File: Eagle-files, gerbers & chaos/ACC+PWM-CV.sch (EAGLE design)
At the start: 57 parts, among them IC1 TL072P, Q1 BC546A, Q2 BC556A, Q3 BC546A, Q4 BC546A, Q5 BC546A, Q6 BC546A, X1 ACC+TRIG, X2 OUT, X3 SUPPLY

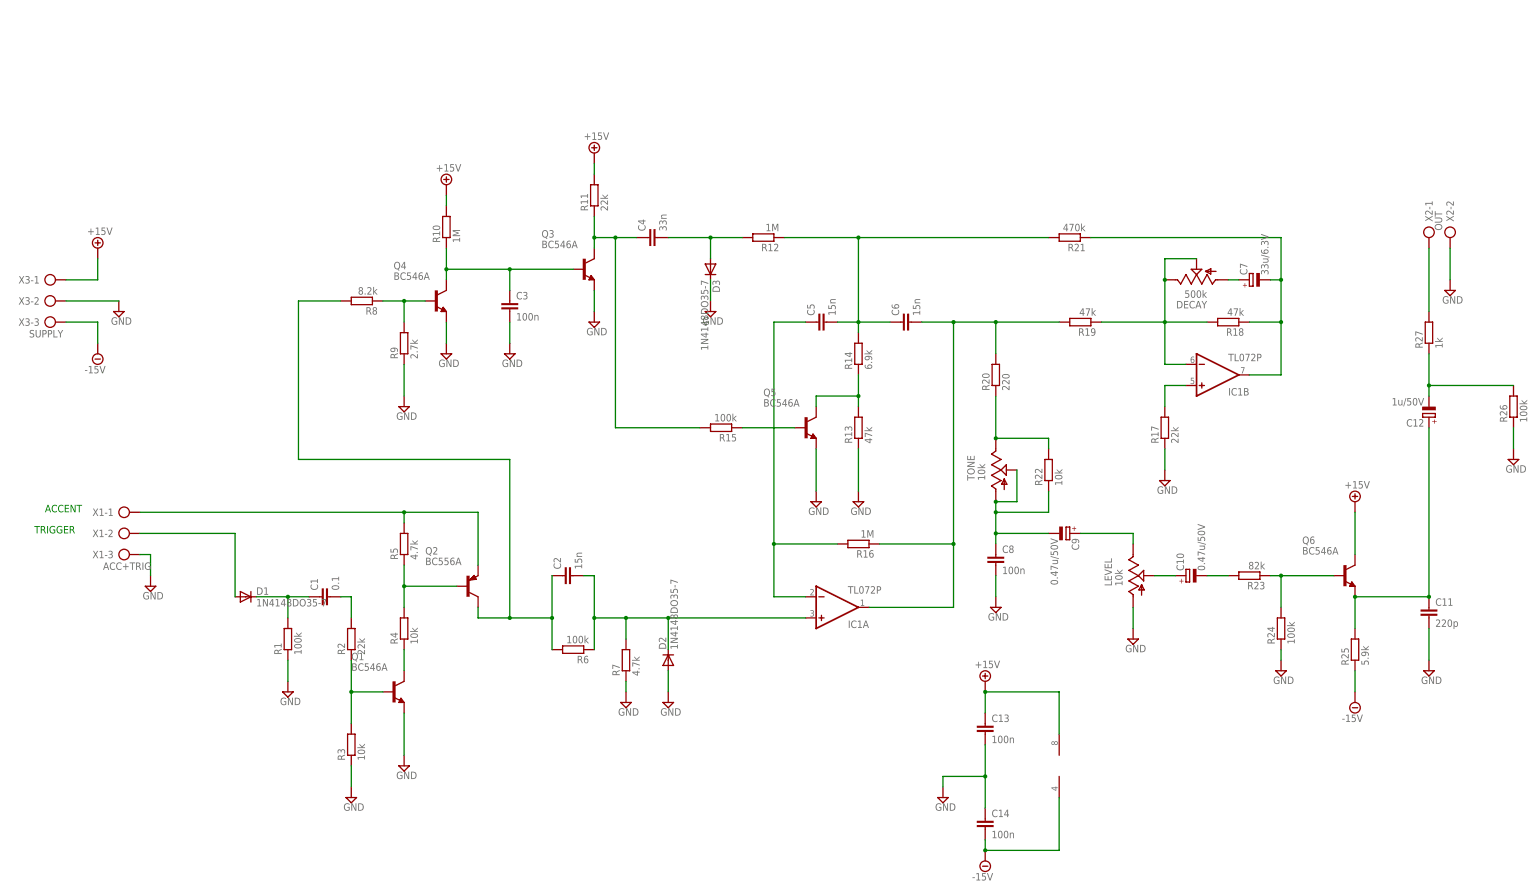
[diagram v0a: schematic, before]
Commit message: Cleaned up, added PDF of schematics
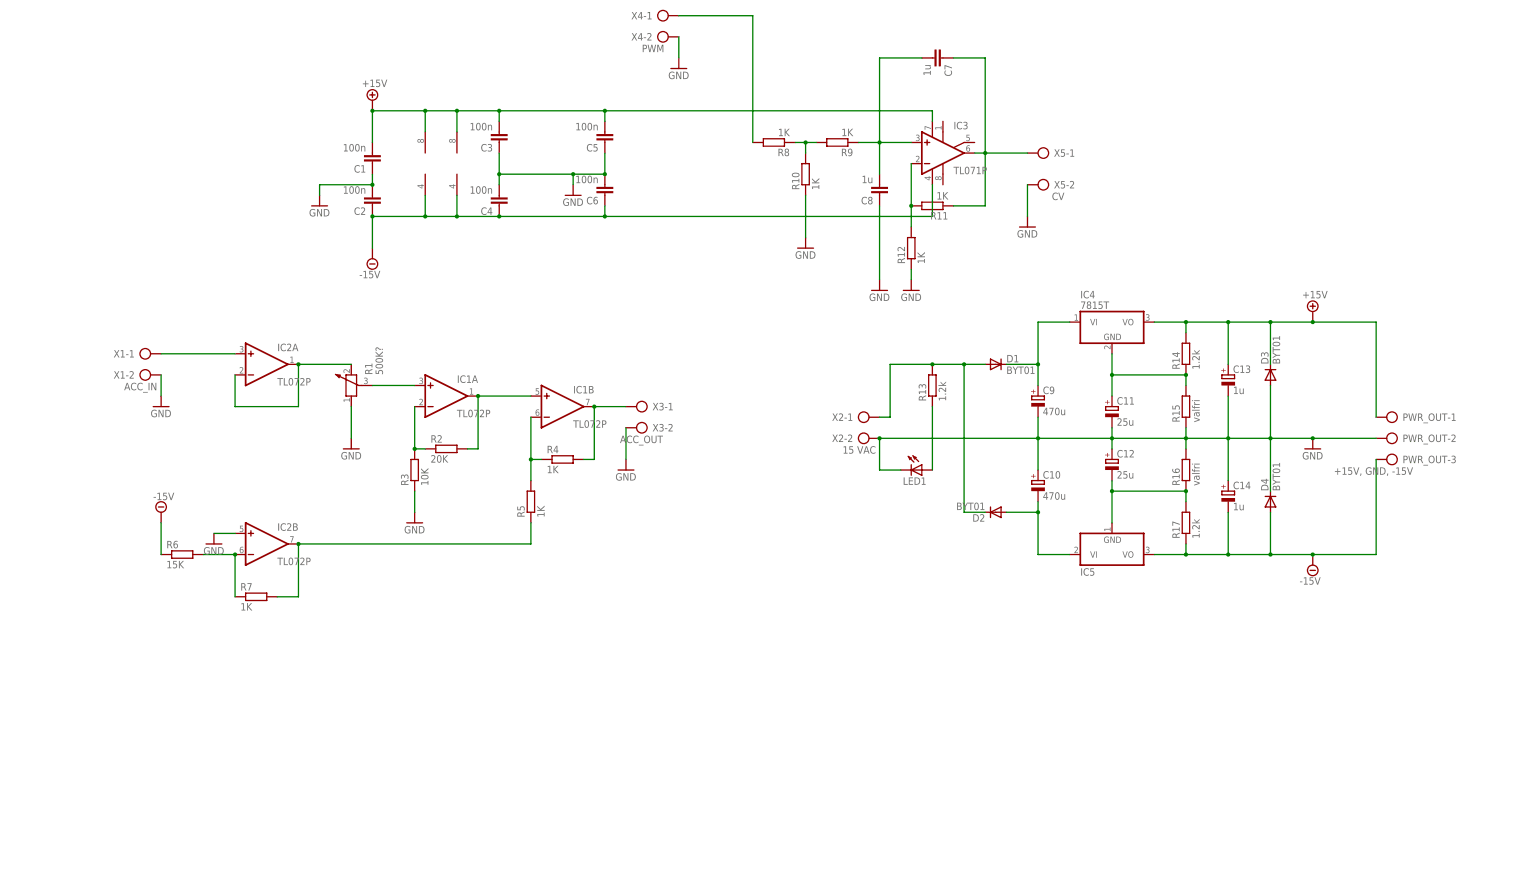
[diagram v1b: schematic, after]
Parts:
- removed DECAY: 500k, pot:TRIM_US-CA9H
- removed LEVEL, TONE: 10k, pot:TRIM_US-CA9H
- removed Q1, Q3, Q4, Q5, Q6: BC546A, transistor-npn:BC546A
- removed Q2: BC556A, transistor-pnp:BC556A
- removed R18, R19: 47k, resistor:R-EU_0207/10
- removed R20: 220, resistor:R-EU_0207/10
- removed R21: 470k, resistor:R-EU_0207/10
- removed R22: 10k, resistor:R-EU_0207/10
- removed R23: 82k, resistor:R-EU_0207/10
- removed R24, R26: 100k, resistor:R-EU_0207/10
- removed R25: 5.9k, resistor:R-EU_0207/10
- removed R27: 1k, resistor:R-EU_0207/10
- added D4: BYT01, diode:BYT01
- added IC2: TL072P, linear:TL072P
- added IC3: TL071P, linear:TL071P
- added IC4: 7815T, linear:7815T
- added IC5: (no value), linear:7915T
- added LED1: (no value), led:LED5MM
- added PWR_OUT: +15V, GND, -15V, con-ptr500:AK300/3
- added X4: PWM, con-ptr500:AK300/2
- added X5: CV, con-ptr500:AK300/2
- C1: value 0.1 -> 100n; device capacitor-wima:C2.5/2 -> rcl:C-EU075-042X103
- C10, C9: value 0.47u/50V -> 470u; device rcl:CPOL-EUE2-5 -> rcl:CPOL-EUE5-6
- C11: value 220p -> 25u; device rcl:C-EU075-042X103 -> rcl:CPOL-EUE5-6
- C12: value 1u/50V -> 25u; device rcl:CPOL-EUE2-5 -> rcl:CPOL-EUE5-6
- C13, C14: value 100n -> 1u; device rcl:C-EU075-042X103 -> rcl:CPOL-EUE5-6
- C2, C5, C6: value 15n -> 100n
- C4: value 33n -> 100n
- C7: value 33u/6.3V -> 1u; device rcl:CPOL-EUE2-5 -> rcl:C-EU075-042X103
- C8: value 100n -> 1u
- D1, D2, D3: value 1N4148DO35-7 -> BYT01; device diode:1N4148DO35-7 -> diode:BYT01
- R1: value 100k -> 500K?; device resistor:R-EU_0207/10 -> rcl:POTENTIOMETER_PT-10
- R10, R12: value 1M -> 1K; device resistor:R-EU_0207/10 -> rcl:R-EU_0207/10
- R11: value 22k -> 1K; device resistor:R-EU_0207/10 -> rcl:R-EU_0207/10
- R13: value 47k -> 1.2k; device resistor:R-EU_0207/10 -> rcl:R-EU_0207/10
- R14: value 6.9k -> 1.2k; device resistor:R-EU_0207/10 -> rcl:R-EU_0207/10
- R15: value 100k -> valfri; device resistor:R-EU_0207/10 -> rcl:R-EU_0207/10
- R16: value 1M -> valfri; device resistor:R-EU_0207/10 -> rcl:R-EU_0207/10
- R17: value 22k -> 1.2k; device resistor:R-EU_0207/10 -> rcl:R-EU_0207/10
- R2: value 22k -> 20K; device resistor:R-EU_0207/10 -> rcl:R-EU_0207/10
- R3: value 10k -> 10K; device resistor:R-EU_0207/10 -> rcl:R-EU_0207/10
- R4: value 10k -> 1K; device resistor:R-EU_0207/10 -> rcl:R-EU_0207/10
- R5, R7: value 4.7k -> 1K; device resistor:R-EU_0207/10 -> rcl:R-EU_0207/10
- R6: value 100k -> 15K; device resistor:R-EU_0207/10 -> rcl:R-EU_0207/10
- R8: value 8.2k -> 1K; device resistor:R-EU_0207/10 -> rcl:R-EU_0207/10
- R9: value 2.7k -> 1K; device resistor:R-EU_0207/10 -> rcl:R-EU_0207/10
- X1: value ACC+TRIG -> ACC_IN; device con-ptr500:AK300/3 -> con-ptr500:AK300/2
- X2: value OUT -> 15 VAC
- X3: value SUPPLY -> ACC_OUT; device con-ptr500:AK300/3 -> con-ptr500:AK300/2
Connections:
- removed net N$15: Q5.B, R15.1
- removed net N$16: Q5.C, R13.2, R14.1
- removed net N$17: IC1B.+IN, R17.2
- removed net N$21: C7.-, IC1B.OUT, R18.1, R21.1
- removed net N$25: C8.1, C9.-, R22.1, TONE.A, TONE.S
- removed net N$27: C10.-, R23.2
- removed net N$28: Q6.B, R23.1, R24.2
- removed net N$29: C9.+, LEVEL.E
- removed net N$30: C11.1, C12.+, Q6.E, R25.2
- removed net N$31: C12.-, R26.2, R27.1
- removed net N$32: R27.2, X2-1.KL
- removed net N$33: C5.2, C6.1, R12.1, R14.2, R21.2
- new net N$23: C10.-, D2.A, IC5.VI
- net +15V: now also C1.2, C13.+, C3.2, C5.2, D3.C, IC2P.V+, IC3.V+, IC4.VO, PWR_OUT-1.KL, R14.2; no longer C13.1, Q6.C, R10.2, R11.2, X3-1.KL
- net -15V: now also C14.-, C2.1, C4.1, C6.1, D4.A, IC2P.V-, IC3.V-, IC5.VO, PWR_OUT-3.KL, R17.1, R6.1; no longer C14.2, R25.1, X3-3.KL
- net GND: now also C1.1, C10.+, C11.-, C12.+, C13.-, C14.+, C2.2, C3.1, C4.2, C5.1, C6.2, C8.1, C9.-, D3.A, D4.C, IC2B.+IN, LED1.C, PWR_OUT-2.KL, R10.1, R12.1, R15.1, R16.2, X1-2.KL, X4-2.KL, X5-2.KL; no longer C11.2, C13.2, C14.1, C3.2, C8.2, D2.A, D3.C, LEVEL.A, Q1.E, Q3.E, Q4.E, Q5.E, R13.1, R17.1, R24.1, R26.1, R7.1, R9.1, X1-3.KL
- net N$1: now also IC2A.-IN, IC2A.OUT, R1.2; no longer Q2.E, R5.2, X1-1.KL
- net N$10: now also R8.2, X4-1.KL; no longer C2.2, D2.C, IC1A.+IN, R6.1, R7.2
- net N$11: now also R10.2; no longer Q4.B
- net N$12: now also C7.2, C8.2, IC3.+IN, R9.1; no longer C4.2, D3.A, R12.2
- net N$13: now also C7.1, IC3.OUT, R11.1, X5-1.KL; no longer C3.1, Q3.B, Q4.C, R10.1
- net N$14: now also IC3.-IN, R11.2, R12.2; no longer C4.1, Q3.C, R11.1, R15.2
- net N$19: now also D1.A, D2.C, R13.2, X2-1.KL; no longer C5.1, IC1A.-IN, R16.2
- net N$2: now also IC1A.+IN, R1.3; no longer C1.1, D1.C, R1.2
- net N$20: now also LED1.A, R13.1; no longer C6.2, IC1A.OUT, R16.1, R19.2, R20.2
- net N$22: now also C9.+, D1.C, IC4.VI; no longer C7.+, DECAY.A
- net N$24: now also C11.+, IC4.GND, R14.1, R15.2; no longer R20.1, R22.2, TONE.E
- net N$26: now also C12.-, IC5.GND, R16.1, R17.2; no longer C10.+, LEVEL.S
- net N$3: now also IC1A.OUT, IC1B.+IN; no longer C1.2
- net N$4: now also IC1A.-IN; no longer Q1.B
- net N$5: now also IC2B.OUT, R5.1, R7.2; no longer DECAY.E, DECAY.S, IC1B.-IN, R18.2, R19.1
- net N$6: now also IC2B.-IN, R6.2, R7.1; no longer Q1.C, R4.1
- net N$7: now also IC1B.-IN, R4.1, R5.2; no longer Q2.B, R4.2, R5.1
- net N$8: now also IC1B.OUT, R4.2, X3-1.KL; no longer D1.A, X1-2.KL
- net N$9: now also IC2A.+IN, X1-1.KL; no longer C2.1, Q2.C, R6.2, R8.2
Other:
- note removed: "ACCENT"
- note removed: "TRIGGER"
- moved on the sheet: C1, C10, C12, C2, C3, C4, C5, C6, C8, C9, IC1A, IC1B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
